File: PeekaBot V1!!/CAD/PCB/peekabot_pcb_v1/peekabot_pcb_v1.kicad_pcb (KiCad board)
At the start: 2 copper layers, 25 parts, among them J1 esp32camright, J2 esp32camleft, J3 USB_B_Micro, J4 Battery Socket, SW1 SW_Push, SW2 SW_Push, U1 IP5306

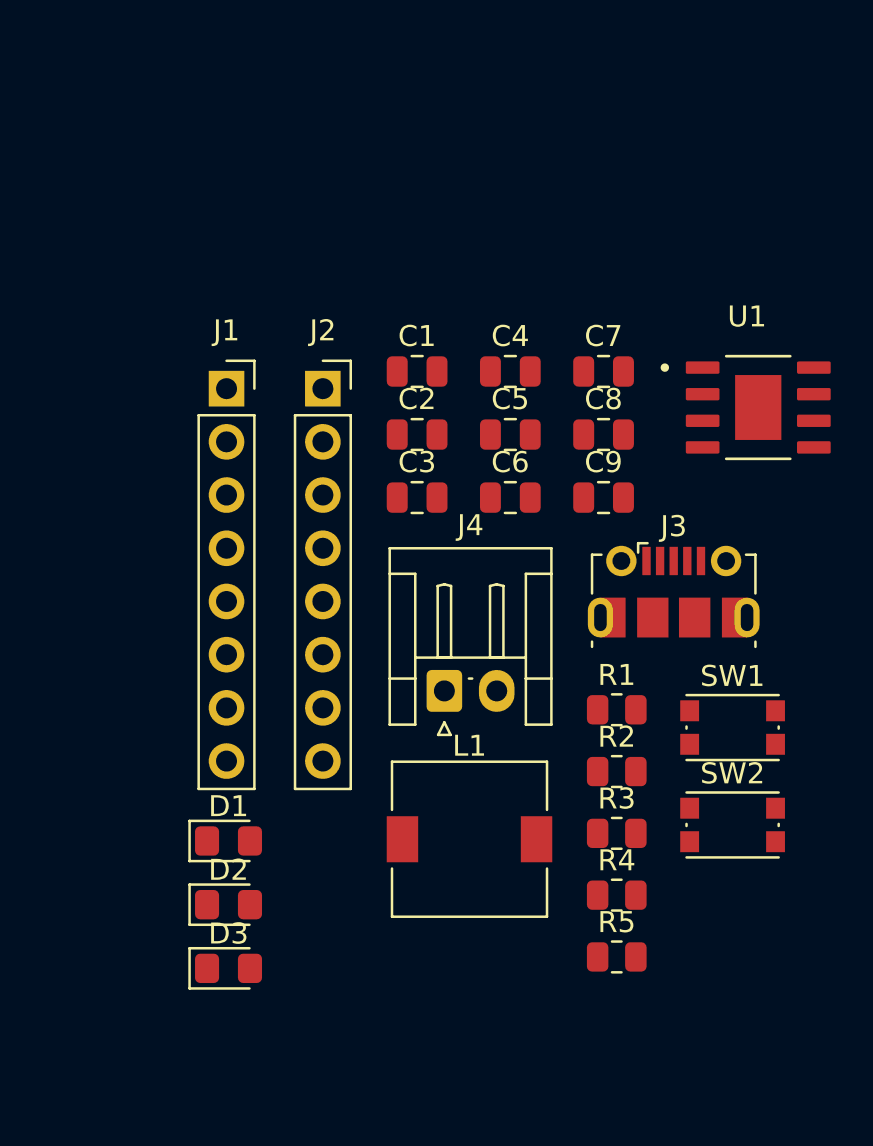
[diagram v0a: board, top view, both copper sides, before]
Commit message: UPDATED PCB-MARK-1!!!
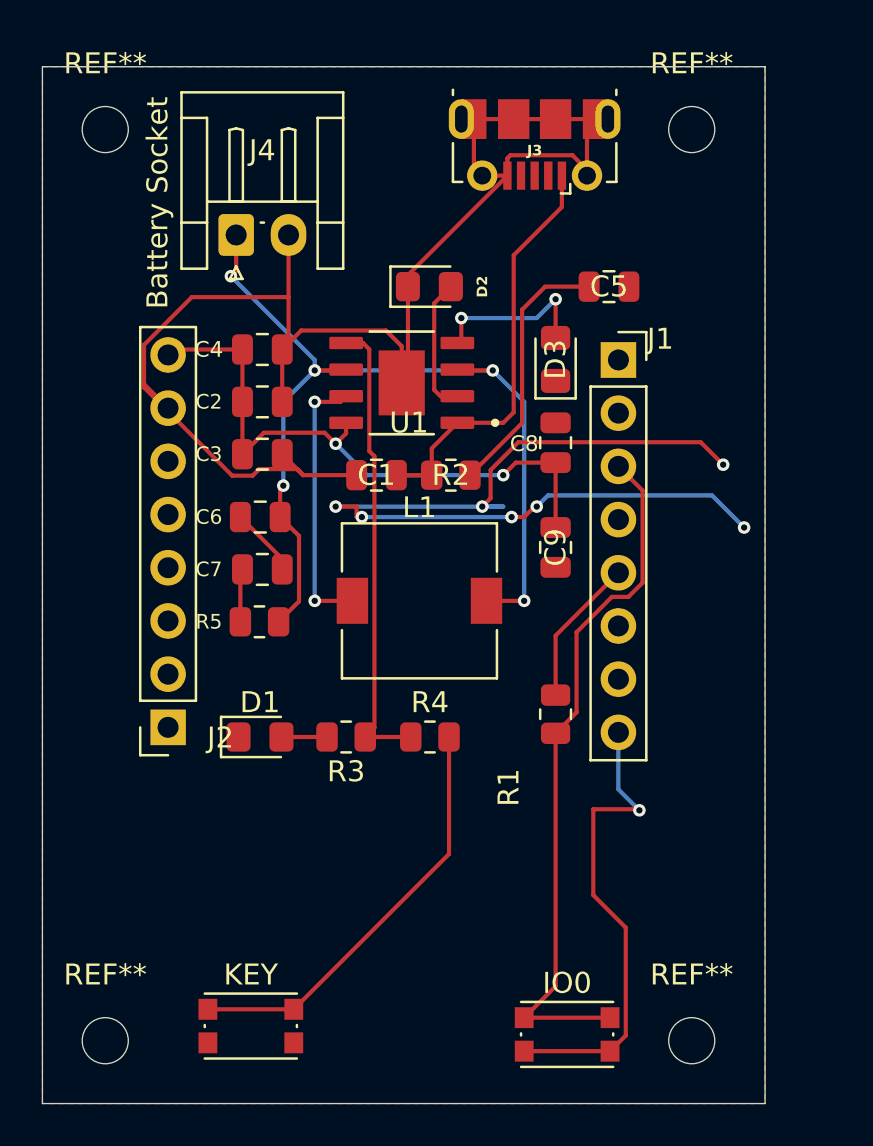
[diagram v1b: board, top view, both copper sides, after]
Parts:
- added REF**: M2, MountingHole:MountingHole_2.2mm_M2, F.Cu at (128.5, 56.0)
- added REF**: M2, MountingHole:MountingHole_2.2mm_M2, F.Cu at (156.5, 56.0)
- added REF**: M2, MountingHole:MountingHole_2.2mm_M2, F.Cu at (128.5, 99.5)
- added REF**: M2, MountingHole:MountingHole_2.2mm_M2, F.Cu at (156.5, 99.5)
- moved D3 33.0 mm to (150.0, 67.0), turned to 90 degrees
- moved D2 31.0 mm to (144.0, 63.5)
- moved KEY 24.9 mm to (135.4, 98.8)
- moved J4 23.9 mm to (134.8, 61.0)
- moved R5 23.4 mm to (135.9, 79.5), turned to 180 degrees
- moved J3 22.3 mm to (149.0, 56.7), turned to 180 degrees
- moved C7 18.8 mm to (136.0, 77.0)
- moved J1 18.8 mm to (153.0, 67.0)
- moved J2 17.8 mm to (131.5, 84.5), turned to 180 degrees
- moved U1 17.1 mm to (142.7, 68.1), turned to 180 degrees
- moved IO0 16.6 mm to (150.6, 99.2)
- moved R2 16.2 mm to (145.0, 72.5)
- moved R3 13.7 mm to (140.0, 85.0), turned to 180 degrees
- moved C6 12.0 mm to (135.9, 74.5), turned to 180 degrees
- moved C4 11.9 mm to (136.0, 66.5)
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- renumbered SW1 to IO0, SW2 to KEY
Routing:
- net GND: track 0.00 -> 99.4 mm, vias 0 -> 1
- net BAT: track 0.00 -> 46.8 mm, vias 0 -> 5
- net (no net): track 0.00 -> 44.9 mm, vias 0 -> 7
- net io0: track 0.00 -> 33.7 mm
- net 5V: track 0.00 -> 29.4 mm, vias 0 -> 2
- net Net-(U1-KEY): track 0.00 -> 22.2 mm
- net Net-(R4-Pad2): track 0.00 -> 20.2 mm
- net Net-(J3-VBUS): track 0.00 -> 19.8 mm
- net Net-(U1-SW): track 0.00 -> 12.9 mm, vias 0 -> 2
- net Net-(C5-Pad1): track 0.00 -> 12.6 mm
- net Net-(D3-A): track 0.00 -> 7.99 mm, vias 0 -> 2
- net VCC: track 0.00 -> 7.08 mm
- net Net-(D2-A): track 0.00 -> 6.49 mm
- net Net-(C7-Pad1): track 0.00 -> 2.54 mm
- net Net-(D1-A): track 0.00 -> 2.18 mm
- added copper zone on F.Cu, net GND
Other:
- board outline added: 34.5 x 49.5 mm
